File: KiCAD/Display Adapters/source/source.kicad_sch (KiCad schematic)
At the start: 5 parts, among them J1 20455-040E-76, J2 47272-0001, J3 XT30PW_2_2_-M.G.B

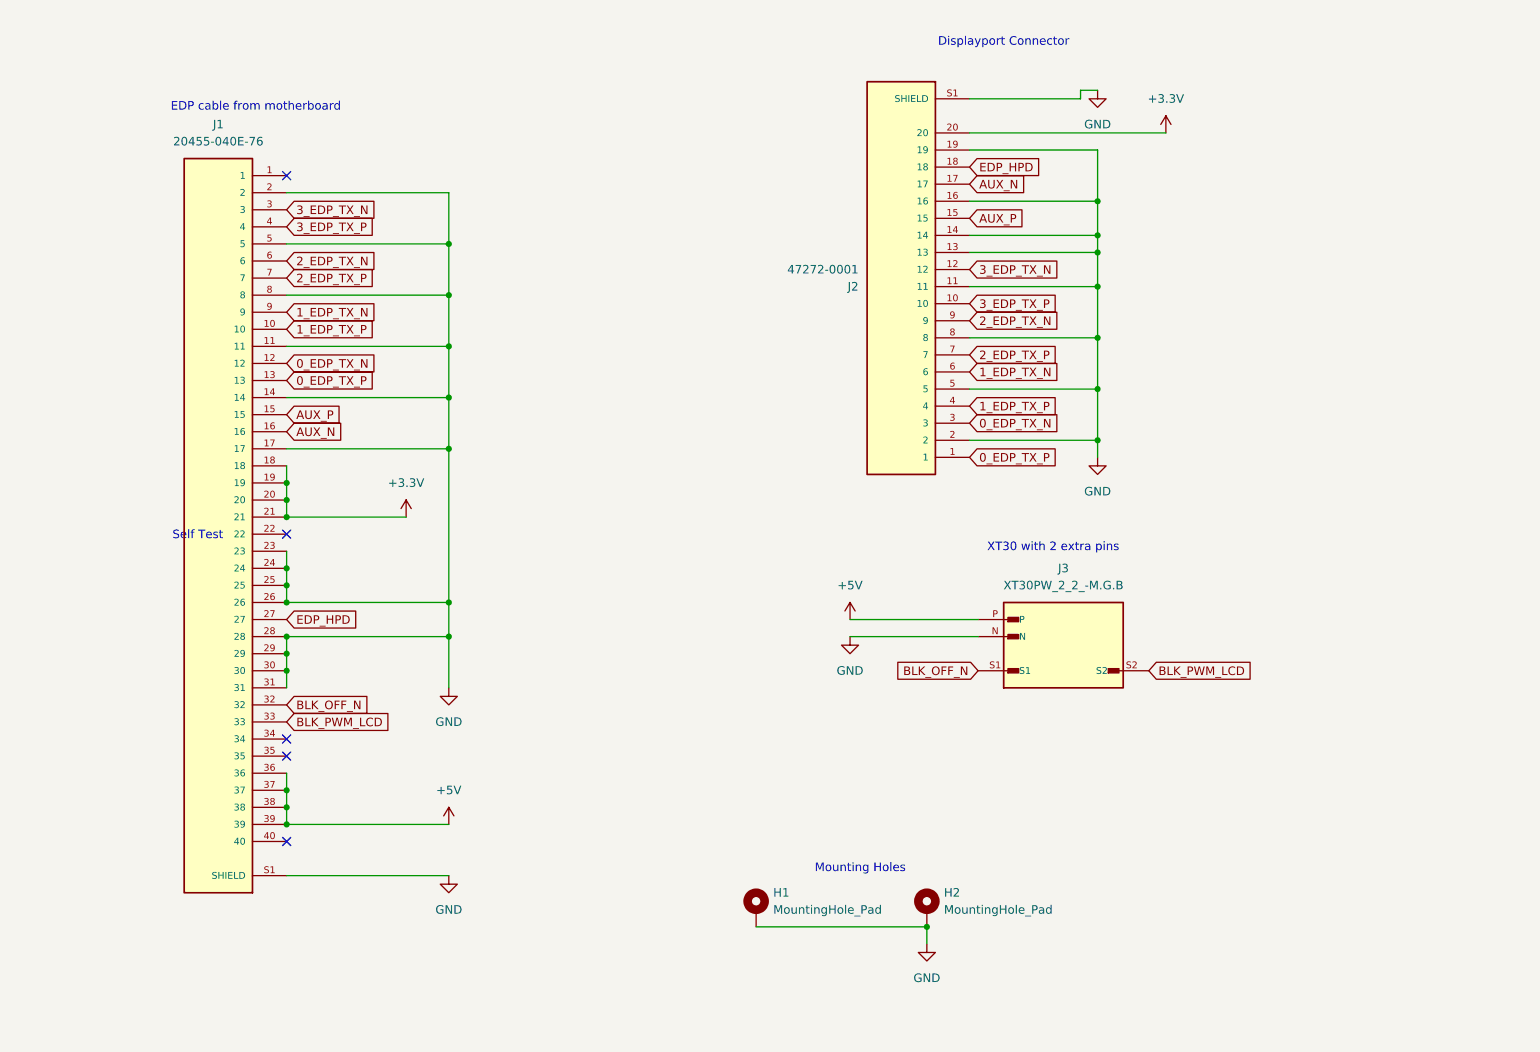
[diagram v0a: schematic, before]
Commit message: fix schematics
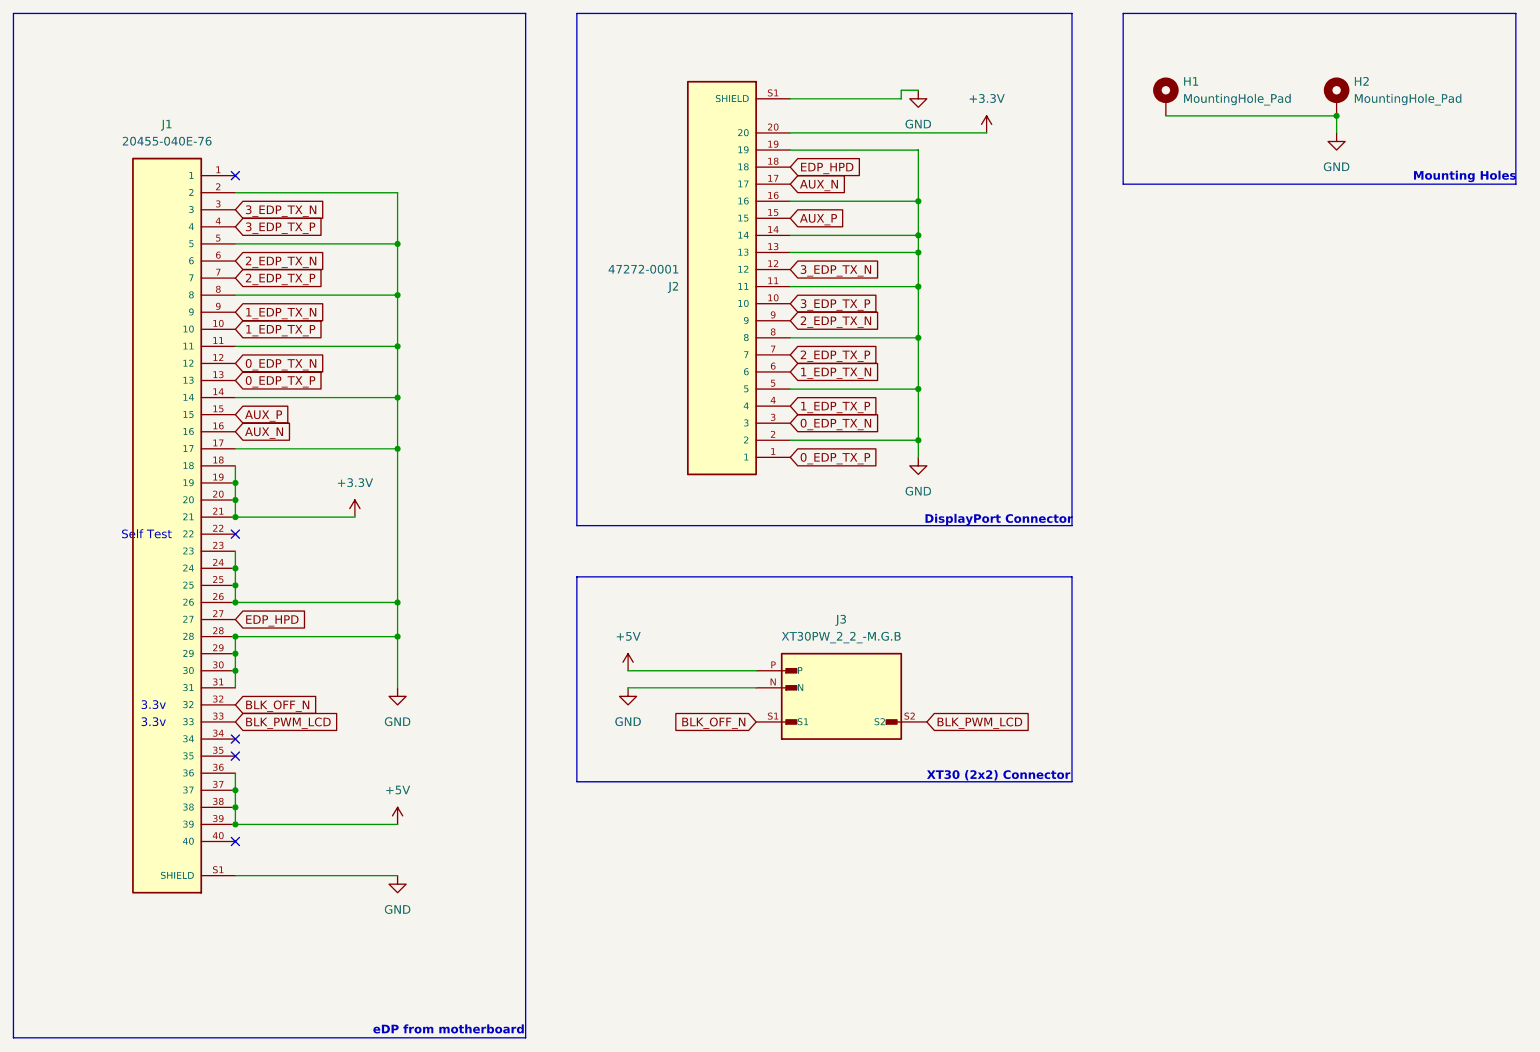
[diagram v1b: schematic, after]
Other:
- note added: "3.3v"
- note added: "DisplayPort Connector"
- note added: "XT30 (2x2) Connector"
- note added: "eDP from motherboard"
- note removed: "Displayport Connector"
- note removed: "EDP cable from motherboard"
- note removed: "XT30 with 2 extra pins"
- title: (none) -> Source: eDP to DP
- moved on the sheet: H1, H2, J1, J2, J3
